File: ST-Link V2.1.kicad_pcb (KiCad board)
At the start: 2 copper layers, 32.1 x 21 mm, 43 parts, among them J1 USB_OTG, J2 Conn_01x06, J3 Conn_01x08, J4 Conn_01x08, Q1 MMBT3904, U1 USBLC6-2SC6, U2 stm32, U3 MIC5219-3.3, X1 8MHz

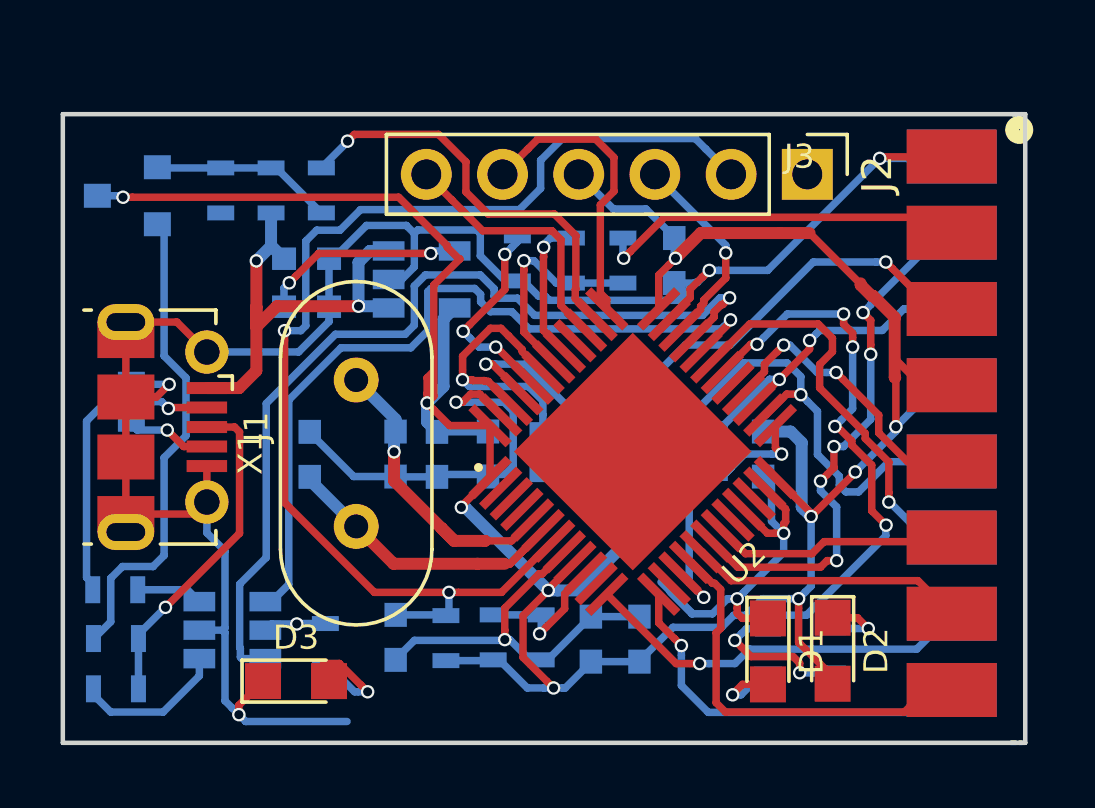
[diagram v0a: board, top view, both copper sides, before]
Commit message: las version need checking
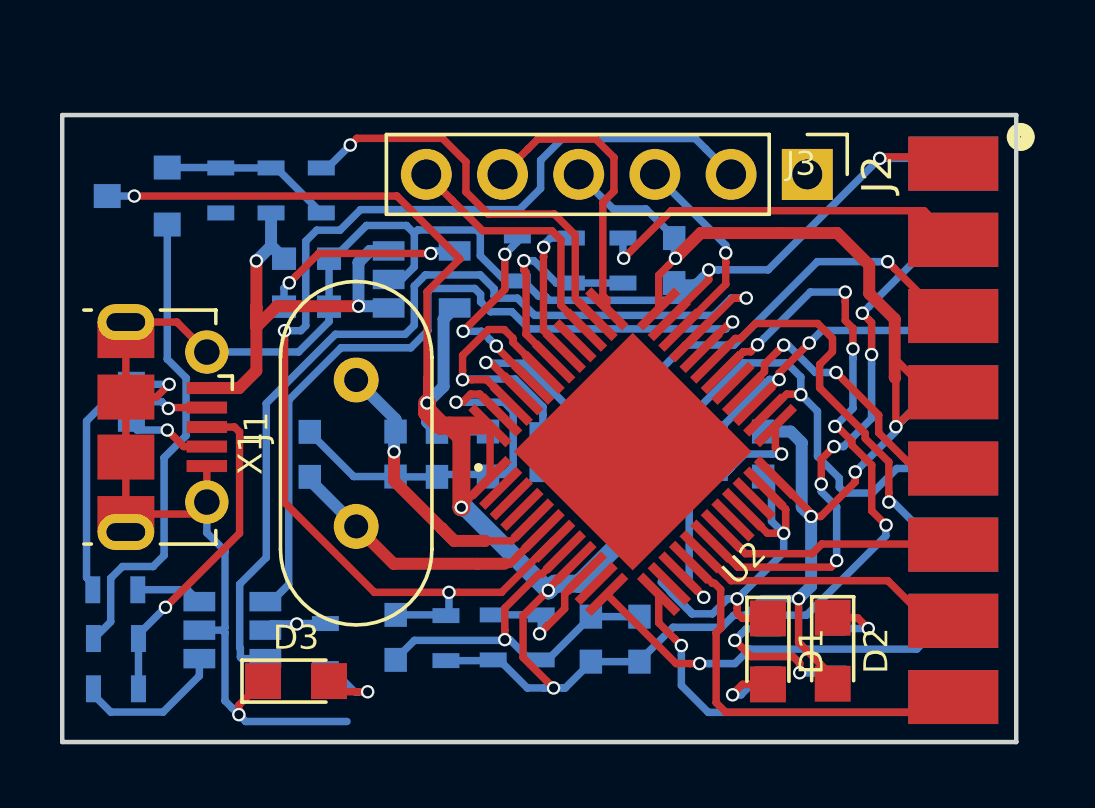
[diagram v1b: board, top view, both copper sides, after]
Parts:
- moved Q1 0.33 mm to (121.2, 100.9)
- moved J3 0.24 mm to (148.4, 99.8)
- moved J4 0.24 mm to (148.4, 99.8)
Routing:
- net /3V3_ST_LINK: track 107.7 -> 117.8 mm
- net /LED_STLINK: track 23.8 -> 24.8 mm
- net /T_RESET: track 12.4 -> 13.5 mm
- net /USB_DP: track 30.6 -> 31.6 mm
- net /T_JTDO: track 13.5 -> 14.3 mm
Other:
- board size 32.1 x 21 mm -> 31.8 x 20.9 mm

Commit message: added label
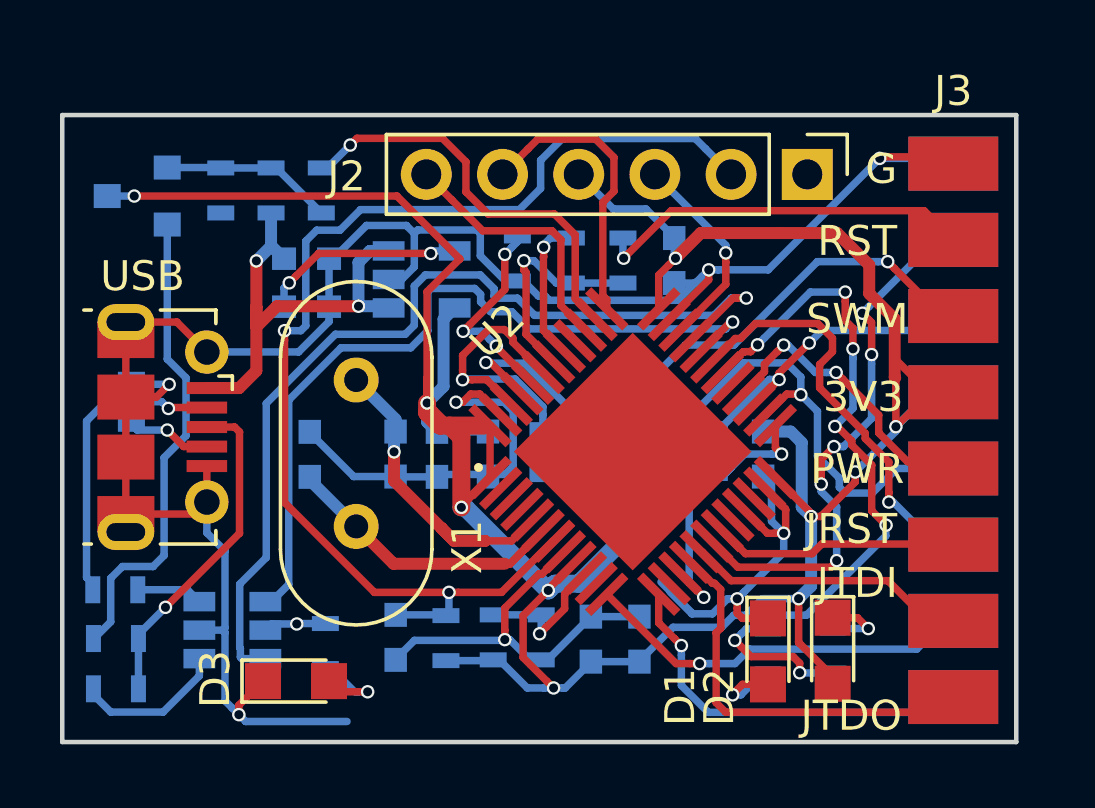
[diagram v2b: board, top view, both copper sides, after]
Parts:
- renumbered J1 to USB
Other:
- board text added: "3V3"
- board text added: "G"
- board text added: "JRST"
- board text added: "JTCK"
- board text added: "JTDI"
- board text added: "JTDO"
- board text added: "JTMS"
- board text added: "PWR"
- board text added: "RST"
- board text added: "RX"
- board text added: "SWM"
- board text added: "SWO"
- board text added: "TX"
- board text added: "nRST"
